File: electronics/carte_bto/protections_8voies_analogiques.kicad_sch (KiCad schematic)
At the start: 40 parts

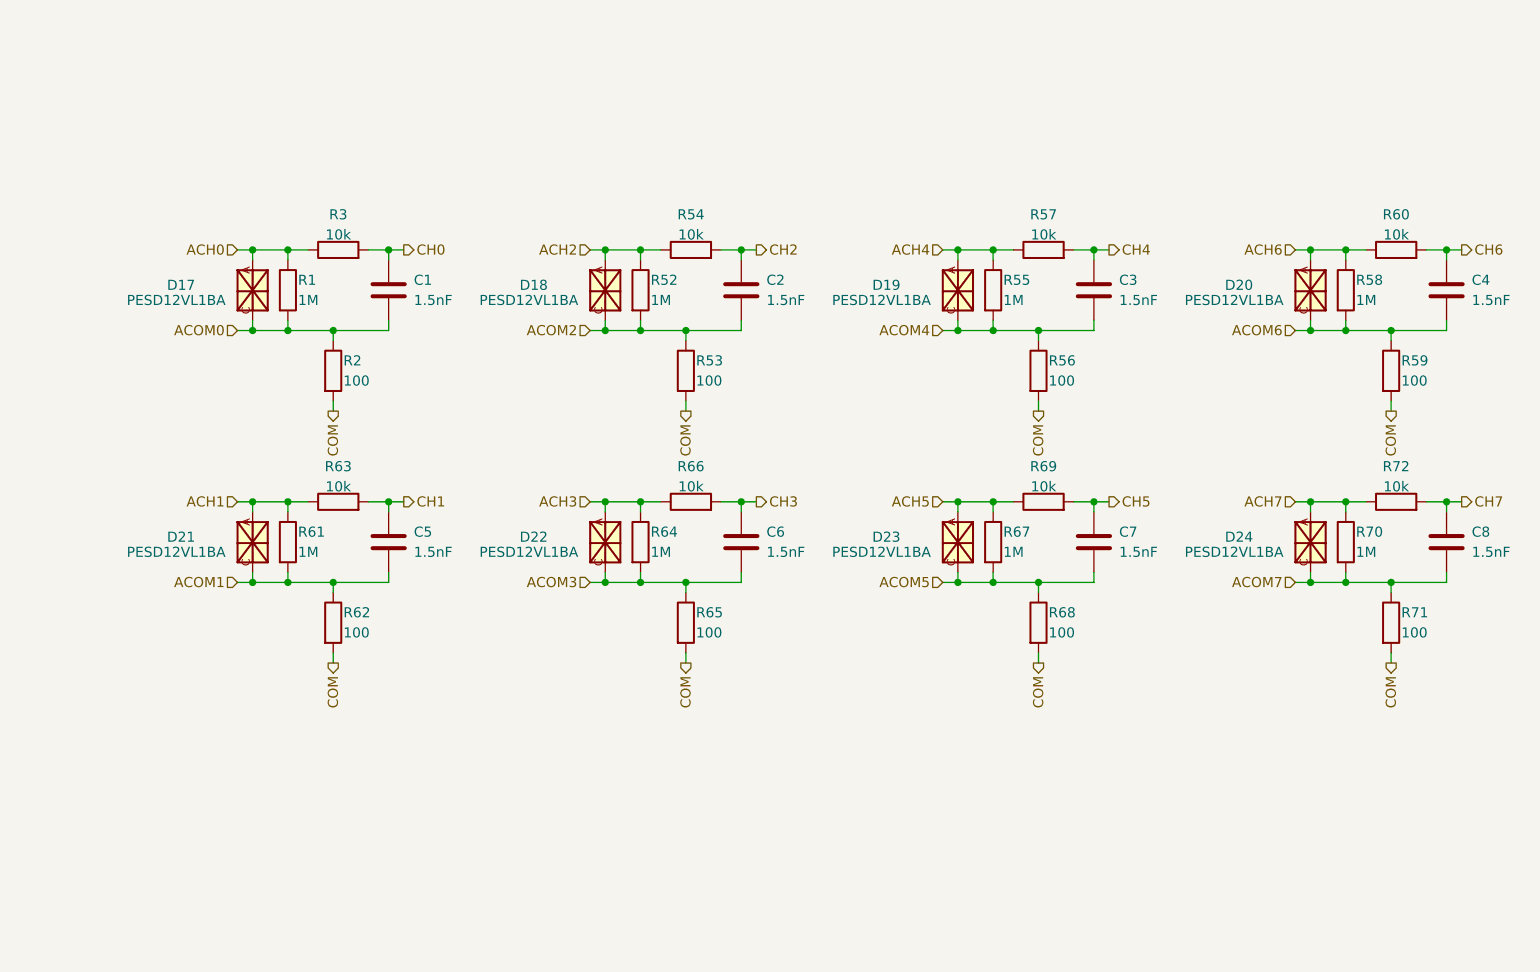
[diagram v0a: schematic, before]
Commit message: BTO schematic: cleanup and documentation
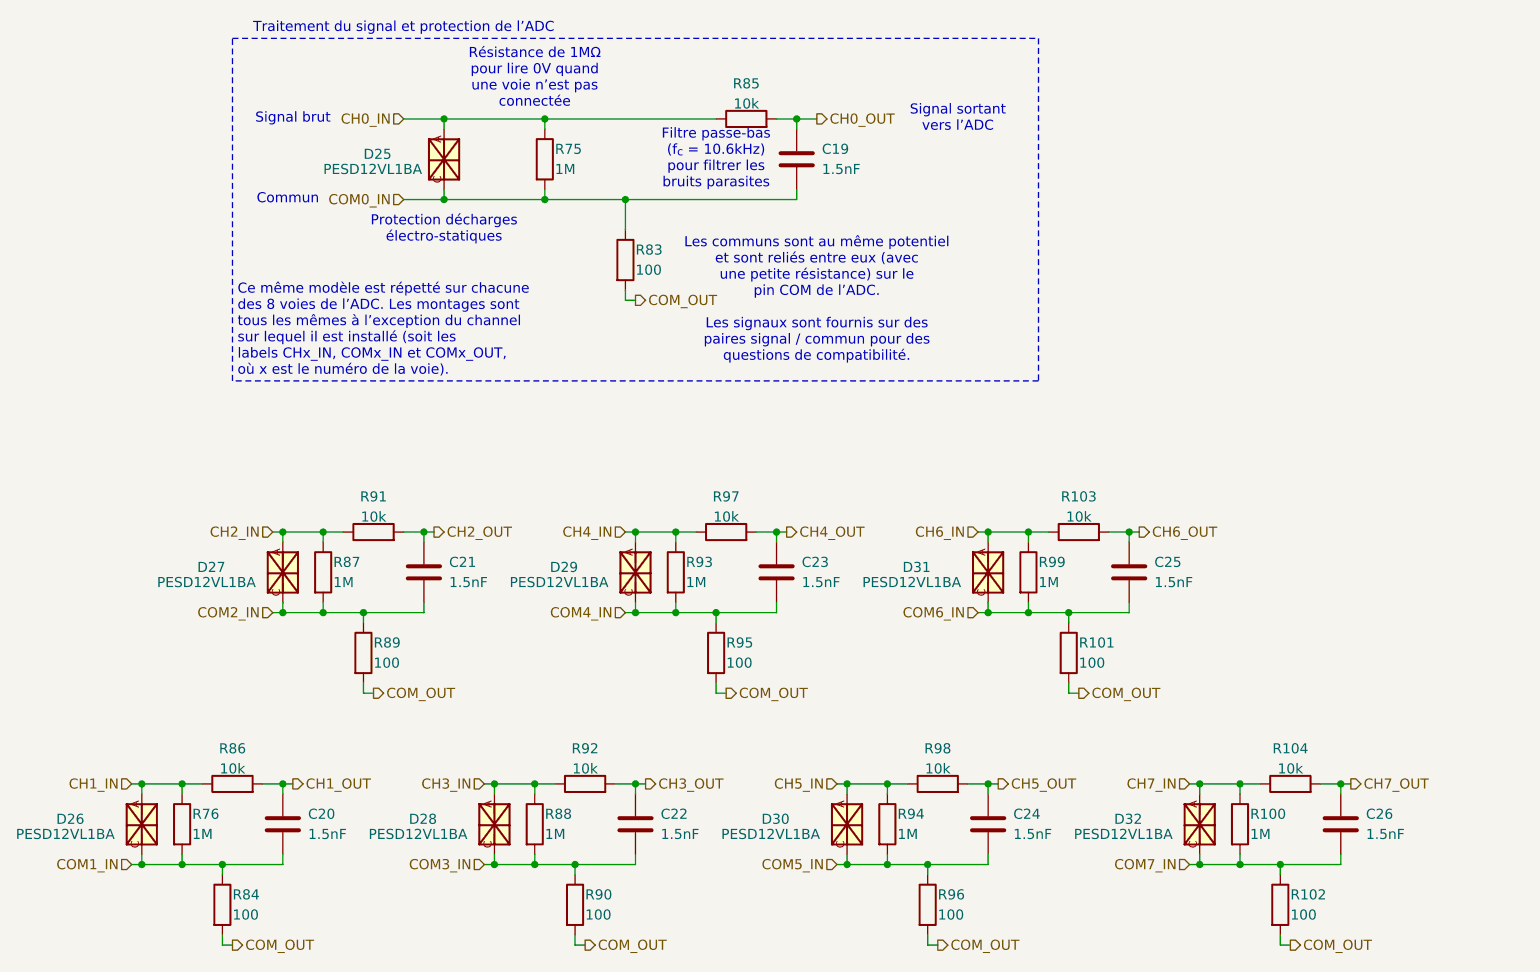
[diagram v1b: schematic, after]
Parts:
- renumbered C1 to C19, C5 to C20, C2 to C21, C6 to C22, C3 to C23, C7 to C24, C4 to C25, C8 to C26, D17 to D25, D21 to D26, D18 to D27, D22 to D28, D19 to D29, D23 to D30, D20 to D31, D24 to D32, R70 to R100, R59 to R101, R71 to R102, R60 to R103, R72 to R104, R1 to R75, R61 to R76, R2 to R83, R62 to R84, R3 to R85, R63 to R86, R52 to R87, R64 to R88, R53 to R89, R65 to R90, R54 to R91, R66 to R92, R55 to R93, R67 to R94, R56 to R95, R68 to R96, R57 to R97, R69 to R98, R58 to R99
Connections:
- net ACH0 renamed CH0_IN
- net ACH1 renamed CH1_IN
- net ACH2 renamed CH2_IN
- net ACH3 renamed CH3_IN
- net ACH4 renamed CH4_IN
- net ACH5 renamed CH5_IN
- net ACH6 renamed CH6_IN
- net ACH7 renamed CH7_IN
- net ACOM0 renamed COM0_IN
- net ACOM1 renamed COM1_IN
- net ACOM2 renamed COM2_IN
- net ACOM3 renamed COM3_IN
- net ACOM4 renamed COM4_IN
- net ACOM5 renamed COM5_IN
- net ACOM6 renamed COM6_IN
- net ACOM7 renamed COM7_IN
- net CH0 renamed CH0_OUT
- net CH1 renamed CH1_OUT
- net CH2 renamed CH2_OUT
- net CH3 renamed CH3_OUT
- net CH4 renamed CH4_OUT
- net CH5 renamed CH5_OUT
- net CH6 renamed CH6_OUT
- net CH7 renamed CH7_OUT
- net COM renamed COM_OUT
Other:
- note added: "Ce même modèle est répetté sur chacune des 8 voies de l’ADC. Les montages sont tous les mêmes à l’exception du channel sur lequel il est installé (soit les labels CHx_IN, COMx_IN et COMx_OUT, où x est le numéro de la voie)."
- note added: "Commun"
- note added: "Filtre passe-bas (f_{c} = 10.6kHz) pour filtrer les bruits parasites"
- note added: "Les communs sont au même potentiel et sont reliés entre eux (avec une petite résistance) sur le pin COM de l’ADC. Les signaux sont fournis sur des paires signal / commun pour des questions de compatibilité."
- note added: "Protection décharges électro-statiques"
- note added: "Résistance de 1MΩ pour lire 0V quand une voie n’est pas connectée"
- note added: "Signal brut"
- note added: "Signal sortant vers l’ADC"
- note added: "Traitement du signal et protection de l’ADC"
- moved on the sheet: C19, C20, C21, C22, C23, C24, C25, C26, D25, D26, D27, D28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
